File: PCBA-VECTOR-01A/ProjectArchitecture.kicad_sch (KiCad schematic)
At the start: 3 parts, among them J10 Conn_02x06_Odd_Even, J11 Conn_02x06_Odd_Even, J9 Conn_02x06_Odd_Even

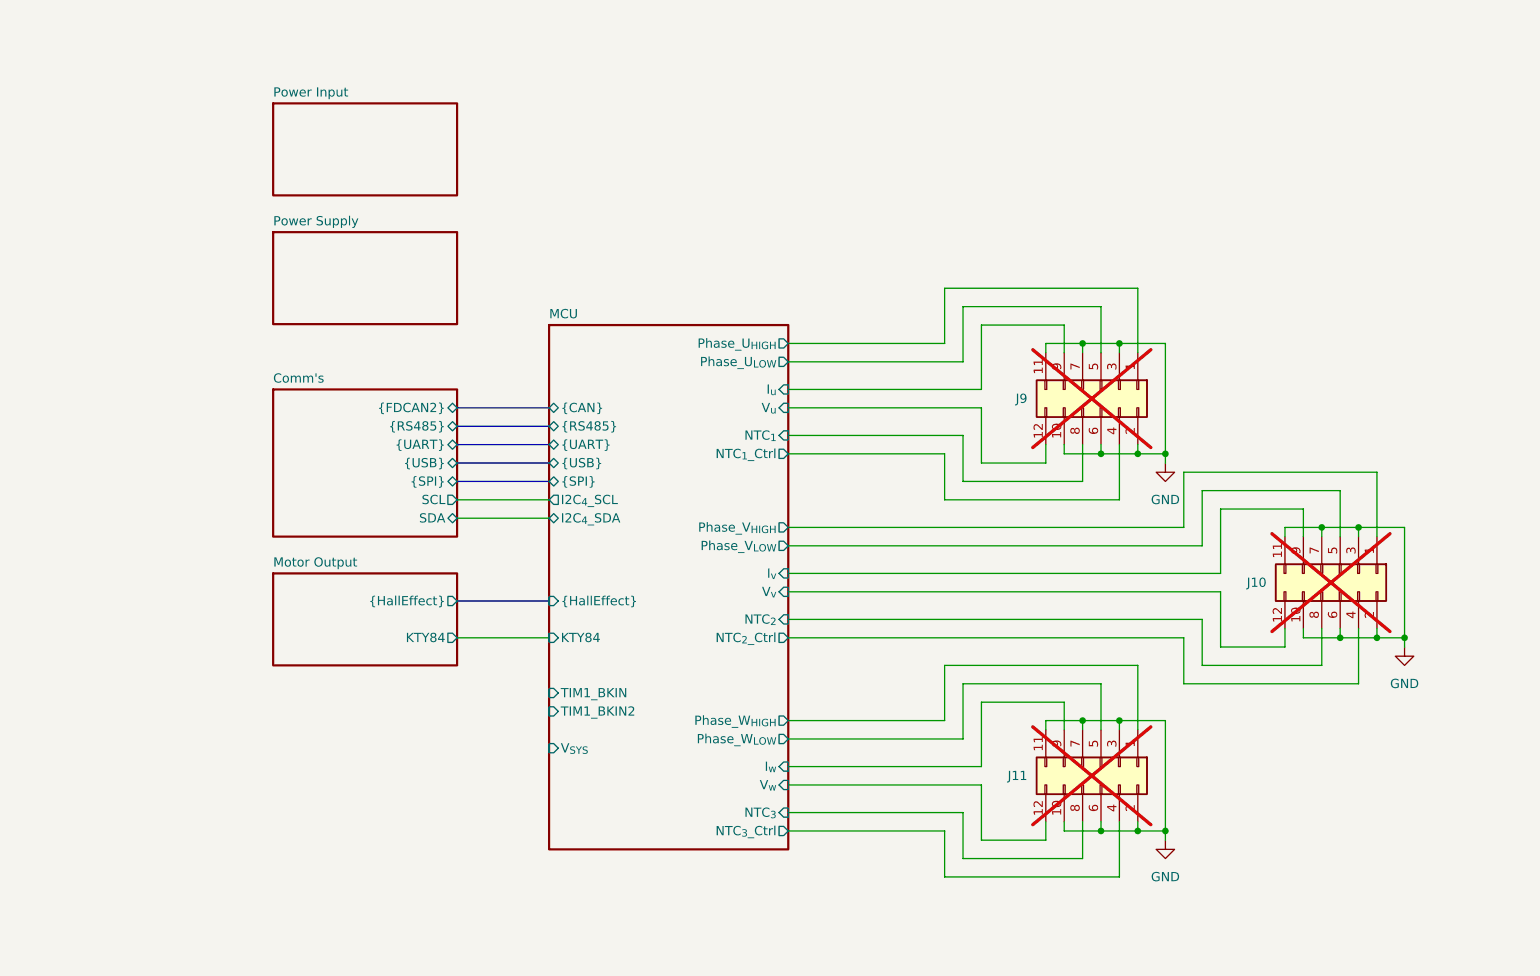
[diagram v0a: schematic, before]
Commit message: Finished schematic?
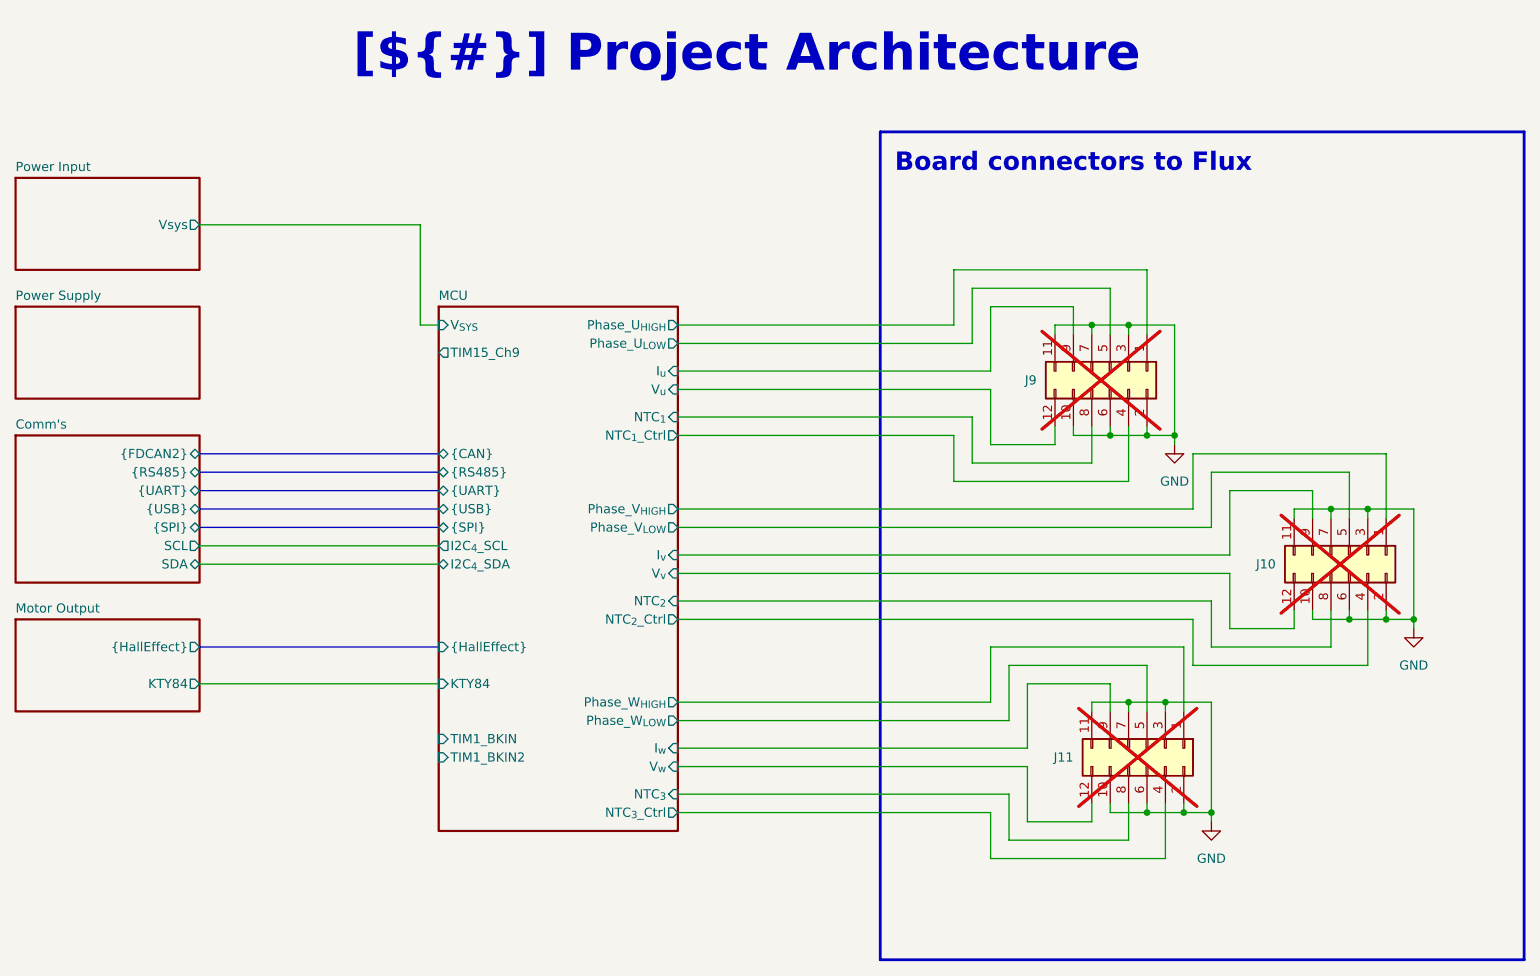
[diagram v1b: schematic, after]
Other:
- sheet MCU ports: added TIM15_Ch9; removed none
- sheet Power Input ports: added Vsys; removed none
- note added: "Board connectors to Flux"
- moved on the sheet: J10, J11, J9
